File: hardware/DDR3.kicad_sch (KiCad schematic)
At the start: 24 parts, among them U1 NT5CB256M16ER-FL

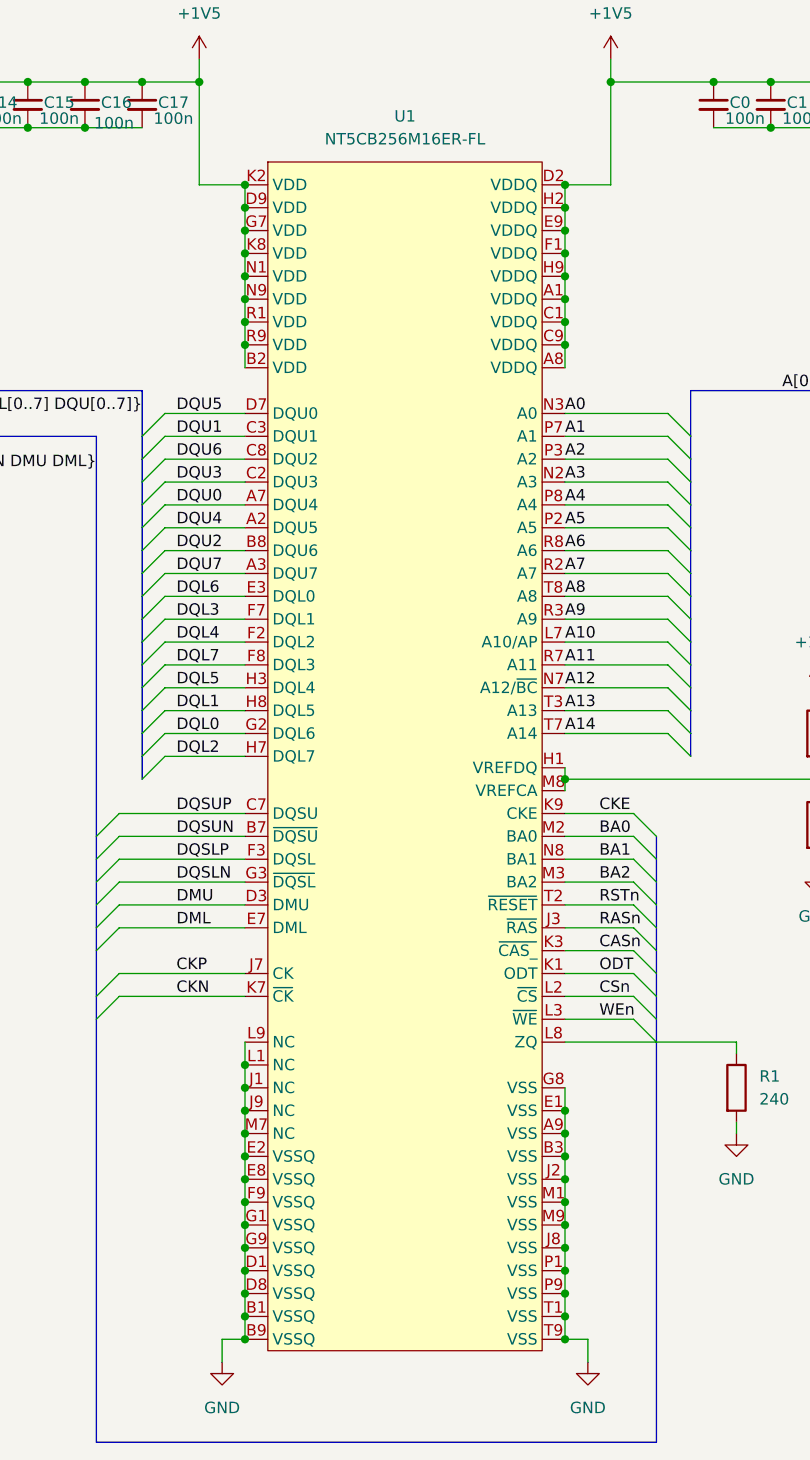
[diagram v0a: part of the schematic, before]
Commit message: stuff
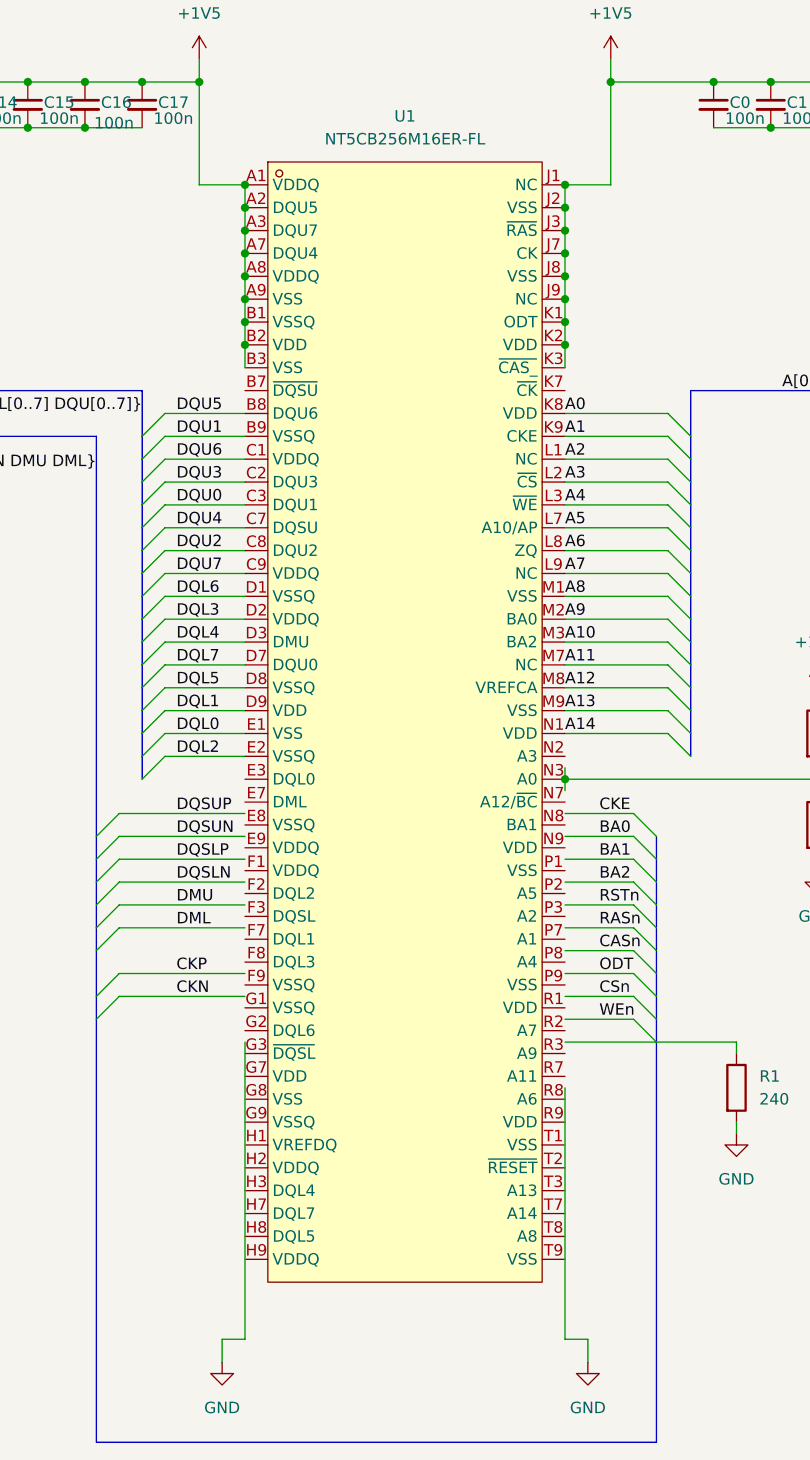
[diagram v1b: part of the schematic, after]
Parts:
- U1: footprint Package_BGA:FBGA-96_8x13mm_Layout9x16_P0.8mm -> easyeda2kicad:TFBGA-96_L13.0-W8.0-R16-C6-P0.80-TL
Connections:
- net +1V5: now also U1.A2 (DQU5), U1.A3 (DQU7), U1.A7 (DQU4), U1.A9 (VSS), U1.B1 (VSSQ), U1.B3 (VSS), U1.J1 (NC), U1.J2 (VSS), U1.J3 (~{RAS}), U1.J7 (CK), U1.J8 (VSS), U1.J9 (NC), U1.K1 (ODT), U1.K3 (~{CAS_}); no longer U1.C1 (VDDQ), U1.C9 (VDDQ), U1.D2 (VDDQ), U1.D9 (VDD), U1.E9 (VDDQ), U1.F1 (VDDQ), U1.G7 (VDD), U1.H2 (VDDQ), U1.H9 (VDDQ), U1.K8 (VDD), U1.N1 (VDD), U1.N9 (VDD), U1.R1 (VDD), U1.R9 (VDD)
- net A0: now also U1.K8 (VDD); no longer U1.N3 (A0)
- net A1: now also U1.K9 (CKE); no longer U1.P7 (A1)
- net A10: now also U1.M3 (BA2); no longer U1.L7 (A10/AP)
- net A11: now also U1.M7 (NC); no longer U1.R7 (A11)
- net A12: now also U1.M8 (VREFCA); no longer U1.N7 (A12/~{BC})
- net A13: now also U1.M9 (VSS); no longer U1.T3 (A13)
- net A14: now also U1.N1 (VDD); no longer U1.T7 (A14)
- net A2: now also U1.L1 (NC); no longer U1.P3 (A2)
- net A3: now also U1.L2 (~{CS}); no longer U1.N2 (A3)
- net A4: now also U1.L3 (~{WE}); no longer U1.P8 (A4)
- net A5: now also U1.L7 (A10/AP); no longer U1.P2 (A5)
- net A6: now also U1.L8 (ZQ); no longer U1.R8 (A6)
- net A7: now also U1.L9 (NC); no longer U1.R2 (A7)
- net A8: now also U1.M1 (VSS); no longer U1.T8 (A8)
- net A9: now also U1.M2 (BA0); no longer U1.R3 (A9)
- net BA0: no longer U1.M2 (BA0)
- net BA1: no longer U1.N8 (BA1)
- net BA2: no longer U1.M3 (BA2)
- net CASn: no longer U1.K3 (~{CAS_})
- net CKE: no longer U1.K9 (CKE)
- net CKN: no longer U1.K7 (~{CK})
- net CKP: no longer U1.J7 (CK)
- net CSn: no longer U1.L2 (~{CS})
- net DML: no longer U1.E7 (DML)
- net DMU: no longer U1.D3 (DMU)
- net DQL0: now also U1.E1 (VSS); no longer U1.G2 (DQL6)
- net DQL1: now also U1.D9 (VDD); no longer U1.H8 (DQL5)
- net DQL2: now also U1.E2 (VSSQ); no longer U1.H7 (DQL7)
- net DQL3: now also U1.D2 (VDDQ); no longer U1.F7 (DQL1)
- net DQL4: now also U1.D3 (DMU); no longer U1.F2 (DQL2)
- net DQL5: now also U1.D8 (VSSQ); no longer U1.H3 (DQL4)
- net DQL6: now also U1.D1 (VSSQ); no longer U1.E3 (DQL0)
- net DQL7: now also U1.D7 (DQU0); no longer U1.F8 (DQL3)
- net DQSLN: no longer U1.G3 (~{DQSL})
- net DQSLP: no longer U1.F3 (DQSL)
- net DQSUN: no longer U1.B7 (~{DQSU})
- net DQSUP: no longer U1.C7 (DQSU)
- net DQU0: now also U1.C3 (DQU1); no longer U1.A7 (DQU4)
- net DQU1: now also U1.B9 (VSSQ); no longer U1.C3 (DQU1)
- net DQU2: now also U1.C8 (DQU2); no longer U1.B8 (DQU6)
- net DQU4: now also U1.C7 (DQSU); no longer U1.A2 (DQU5)
- net DQU5: now also U1.B8 (DQU6); no longer U1.D7 (DQU0)
- net DQU6: now also U1.C1 (VDDQ); no longer U1.C8 (DQU2)
- net DQU7: now also U1.C9 (VDDQ); no longer U1.A3 (DQU7)
- net GND: no longer U1.A9 (VSS), U1.B1 (VSSQ), U1.B3 (VSS), U1.B9 (VSSQ), U1.D1 (VSSQ), U1.D8 (VSSQ), U1.E1 (VSS), U1.E2 (VSSQ), U1.E8 (VSSQ), U1.F9 (VSSQ), U1.G1 (VSSQ), U1.G8 (VSS), U1.G9 (VSSQ), U1.J1 (NC), U1.J2 (VSS), U1.J8 (VSS), U1.J9 (NC), U1.L1 (NC), U1.L9 (NC), U1.M1 (VSS), U1.M7 (NC), U1.M9 (VSS), U1.P1 (VSS), U1.P9 (VSS), U1.T1 (VSS), U1.T9 (VSS)
- net ODT: no longer U1.K1 (ODT)
- net RASn: no longer U1.J3 (~{RAS})
- net RSTn: no longer U1.T2 (~{RESET})
- net WEn: no longer U1.L3 (~{WE})
- net at C18.2, C19.1, R2.2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: now also U1.N3 (A0); no longer U1.H1 (VREFDQ), U1.M8 (VREFCA)
- net at R1.1: no longer U1.L8 (ZQ)
